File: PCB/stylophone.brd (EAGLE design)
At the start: 100 x 73.7 mm, 25 parts, among them IC2 LM358N

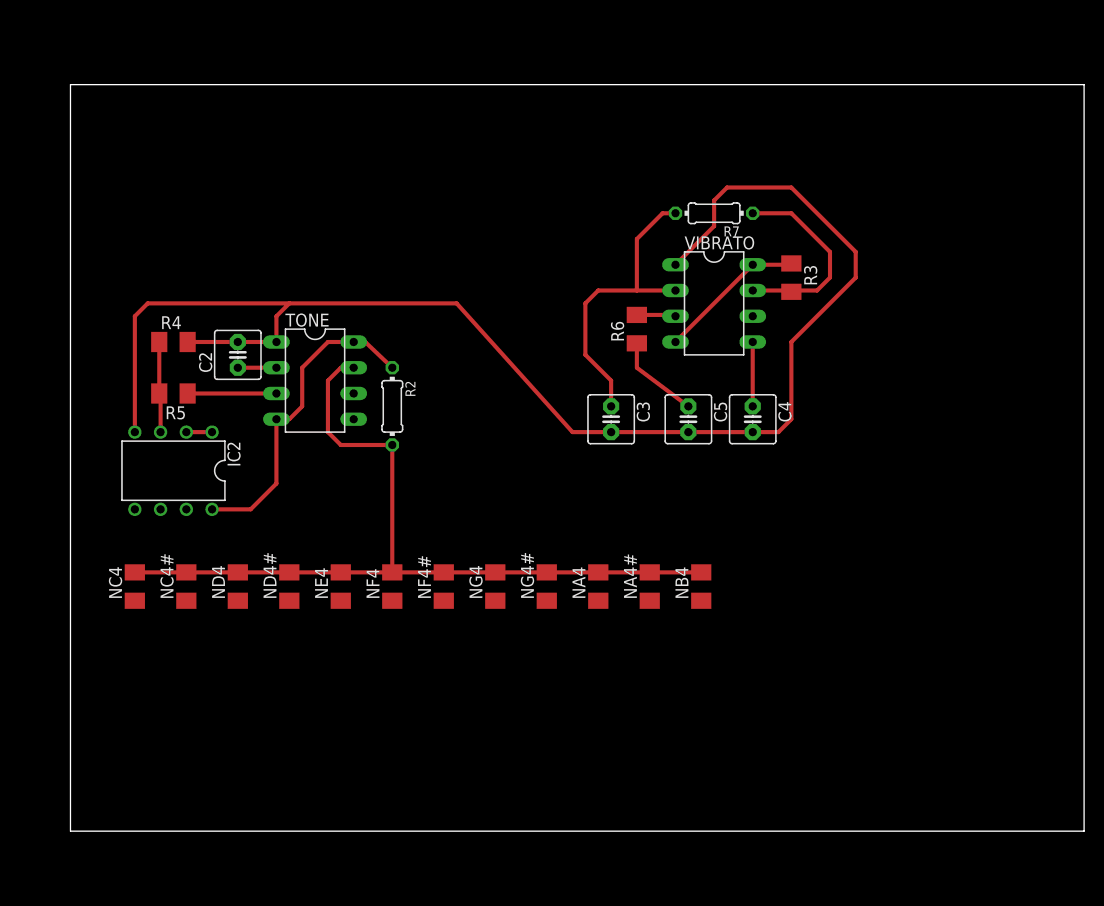
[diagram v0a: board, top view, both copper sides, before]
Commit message: v2
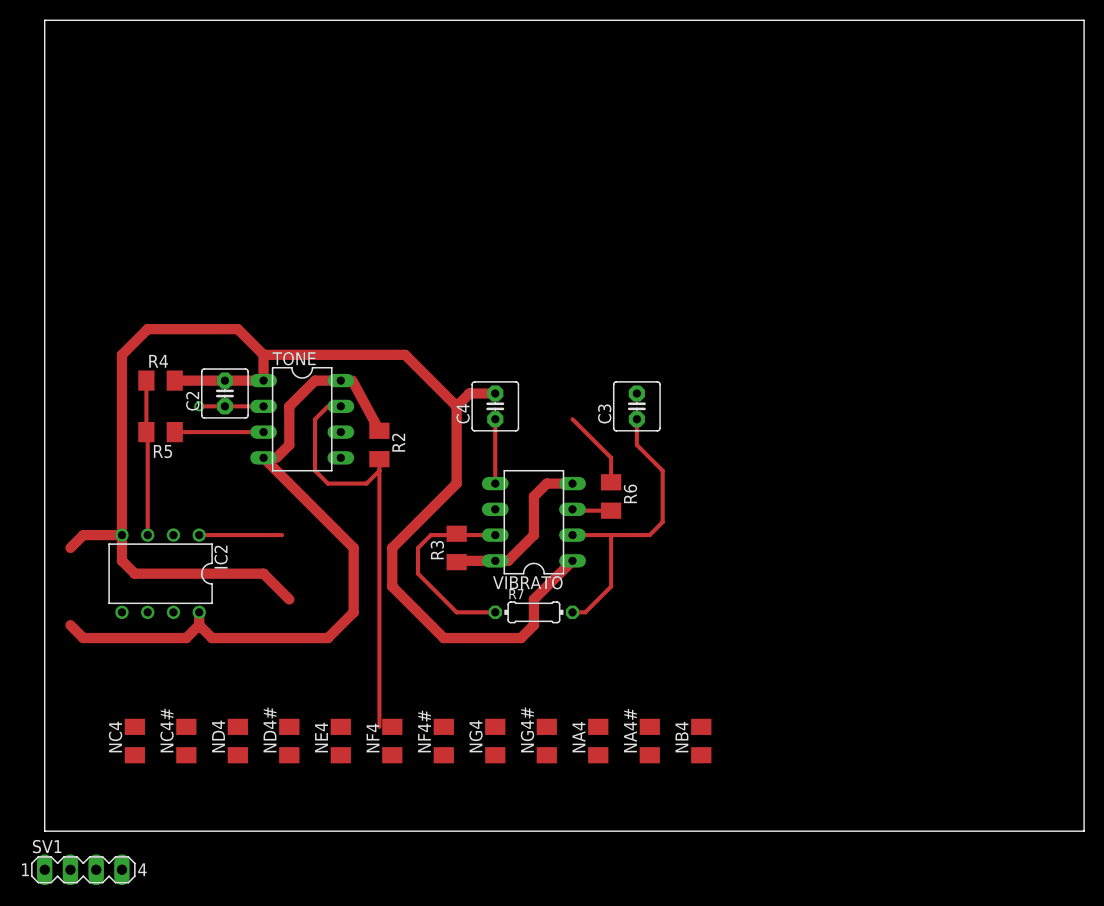
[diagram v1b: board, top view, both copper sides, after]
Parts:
- removed C5: 10u, capacitor-wima:C2.5-5
- added SV1: (no value), con-lstb:MA04-1
- R2: device resistor:0204/7 -> resistor:M1206
- moved R7 43.2 mm to (45.7, 21.6), turned to 0 degrees
- moved R3 42.4 mm to (38.1, 27.9), turned to 90 degrees
- moved VIBRATO 28.0 mm to (45.7, 30.5), turned to 90 degrees
- moved C4 25.4 mm to (41.9, 41.9), turned to 90 degrees
- moved R6 16.7 mm to (53.3, 33.0), turned to 270 degrees
- moved NA4 15.2 mm to (52.1, 8.89)
- moved NA4# 15.2 mm to (57.1, 8.89)
- moved NB4 15.2 mm to (62.2, 8.89)
- moved NC4 15.2 mm to (6.35, 8.89)
- moved NC4# 15.2 mm to (11.4, 8.89)
- moved ND4 15.2 mm to (16.5, 8.89)
- moved ND4# 15.2 mm to (21.6, 8.89)
- moved NE4 15.2 mm to (26.7, 8.89)
- moved NF4 15.2 mm to (31.8, 8.89)
- moved NF4# 15.2 mm to (36.8, 8.89)
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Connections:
- net GND: now also SV1.2, SV1.4; no longer C5.2
- net OUTPUT: now also SV1.3
- net VCC: now also SV1.1
- net VIBRATO: no longer C5.1
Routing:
- net NOTE: track 83.6 -> 40.7 mm
- net VCC: track 46.2 -> 87.4 mm
- net N$5: track 8.94 -> 15.3 mm
- net OUTPUT: track 2.54 -> 8.18 mm
- net STYLUS: track 3.81 -> 6.35 mm, vias 0 -> 1
- net GND: track 140.2 -> 141.8 mm
- net VIBRATO: track 8.76 -> 7.80 mm
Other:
- board size 100 x 73.7 mm -> 102.5 x 80 mm
